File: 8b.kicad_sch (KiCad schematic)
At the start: 60 parts, among them J1 AudioJack2, J11 AudioJack3, J2 AudioJack2, J3 AudioJack2, J4 AudioJack2, J5 AudioJack2, J6 AudioJack2, J7 AudioJack2, J8 AudioJack2, J9 AudioJack3, Q1 2N3904, Q2 2N3904, Q3 2N3904, Q4 2N3904, Q5 2N3904, Q6 2N3904, Q7 2N3904, Q8 2N3904, SW1 SW_Push, SW2 SW_Push, SW3 SW_Push, SW4 SW_Push, SW5 SW_Push, SW6 SW_Push, SW7 SW_Push, SW8 SW_Push, SW9 SW_Push_DPDT

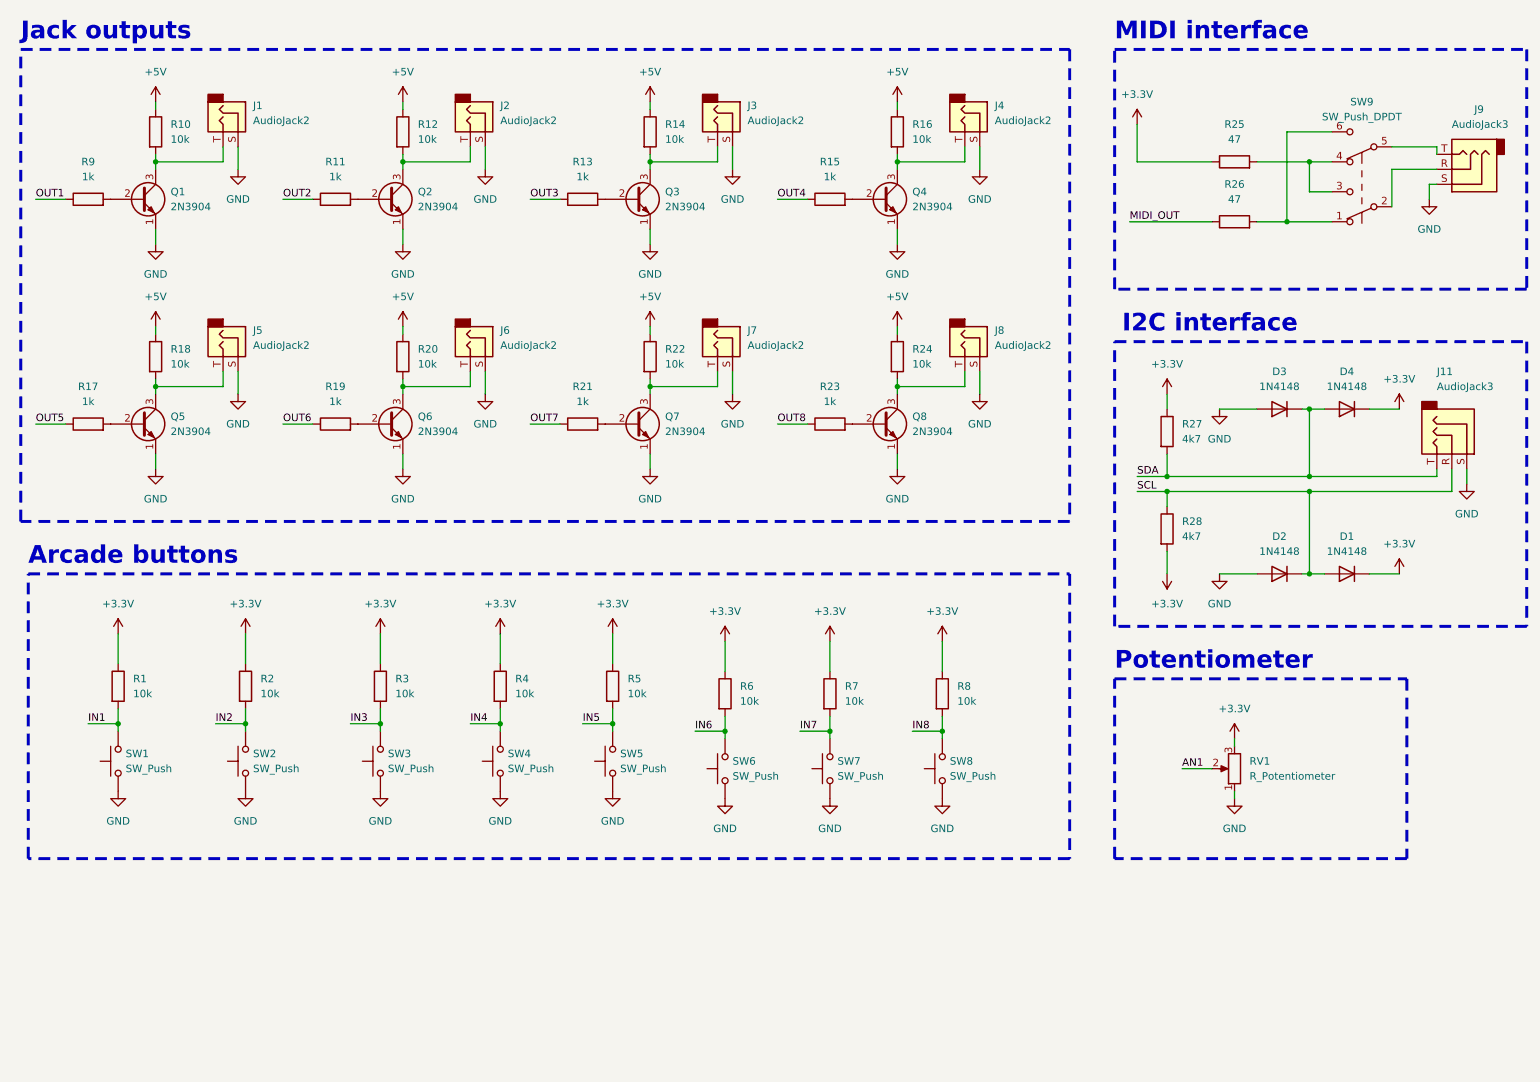
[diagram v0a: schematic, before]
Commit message: Update schem
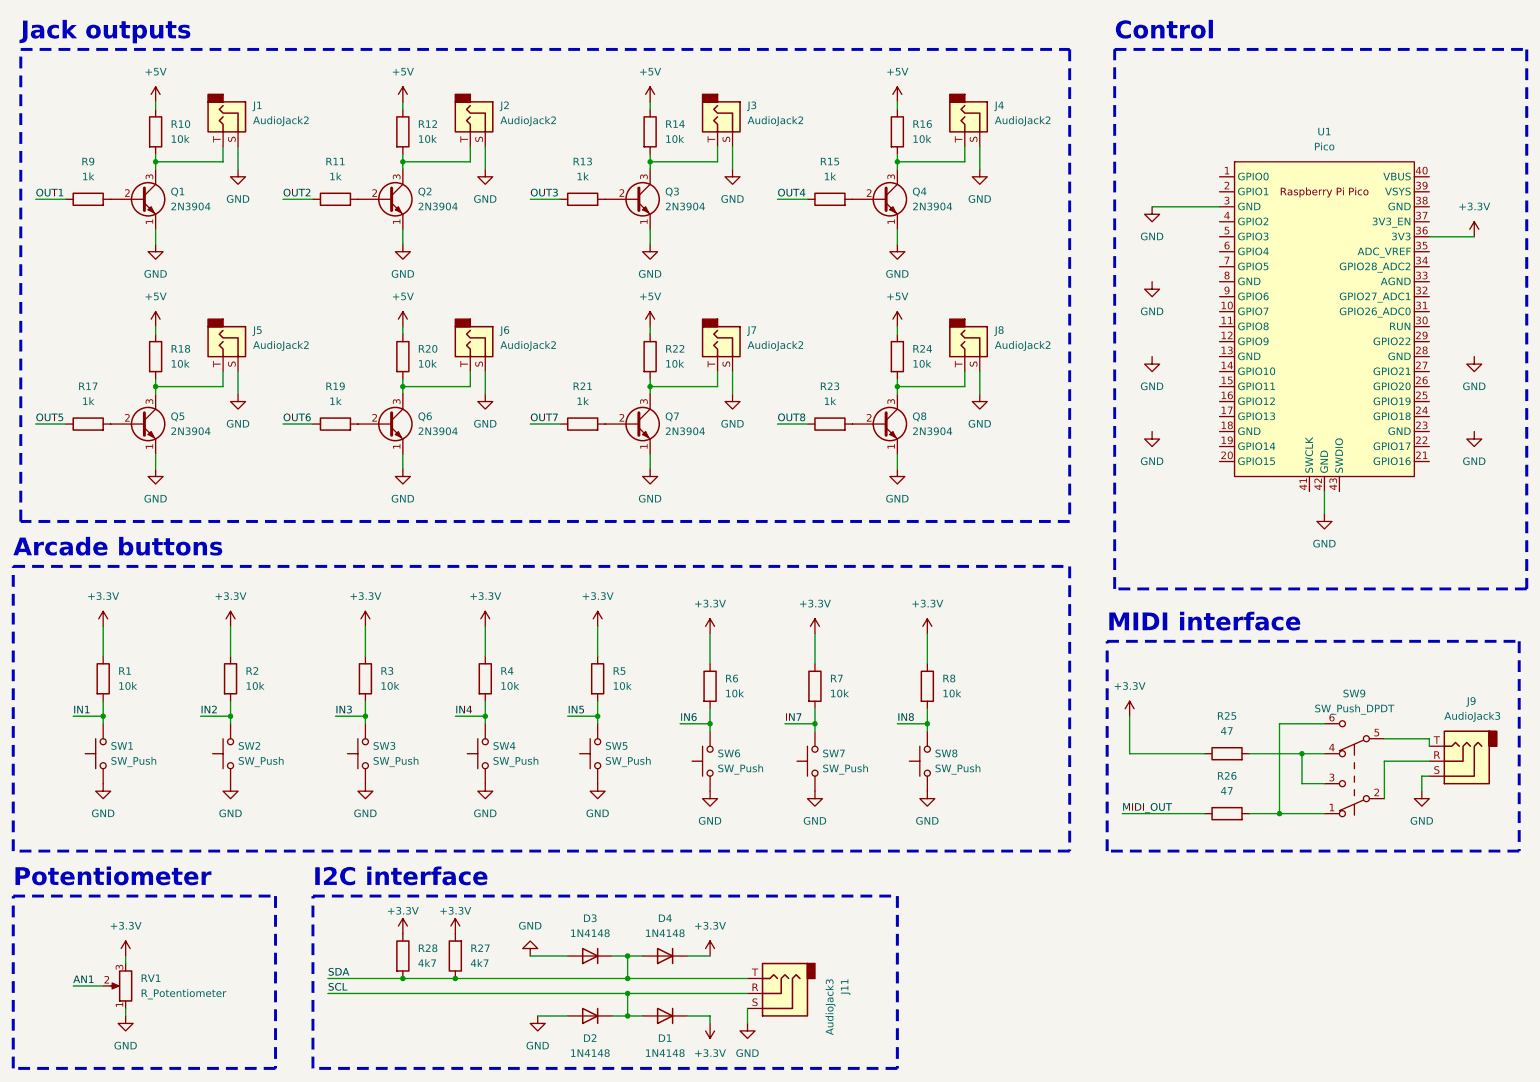
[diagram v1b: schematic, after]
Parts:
- added U1: Pico, RPi_Pico:RPi_Pico_SMD_TH, symbol RPi Pico:Pico
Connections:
- net +3.3V: now also R27.2, R28.1, U1.36 (3V3); no longer R27.1, R28.2
- net GND: now also U1.3 (GND), U1.42 (GND)
- net SCL: no longer R28.1
- net SDA: now also R27.1, R28.2; no longer R27.2
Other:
- note added: "Control"
- moved on the sheet: D1, D2, D3, D4, J11, J9, R1, R2, R25, R26, R27, R28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
